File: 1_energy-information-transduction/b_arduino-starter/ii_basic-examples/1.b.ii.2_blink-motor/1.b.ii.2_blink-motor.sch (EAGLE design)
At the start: 2 parts, among them T1 2N706

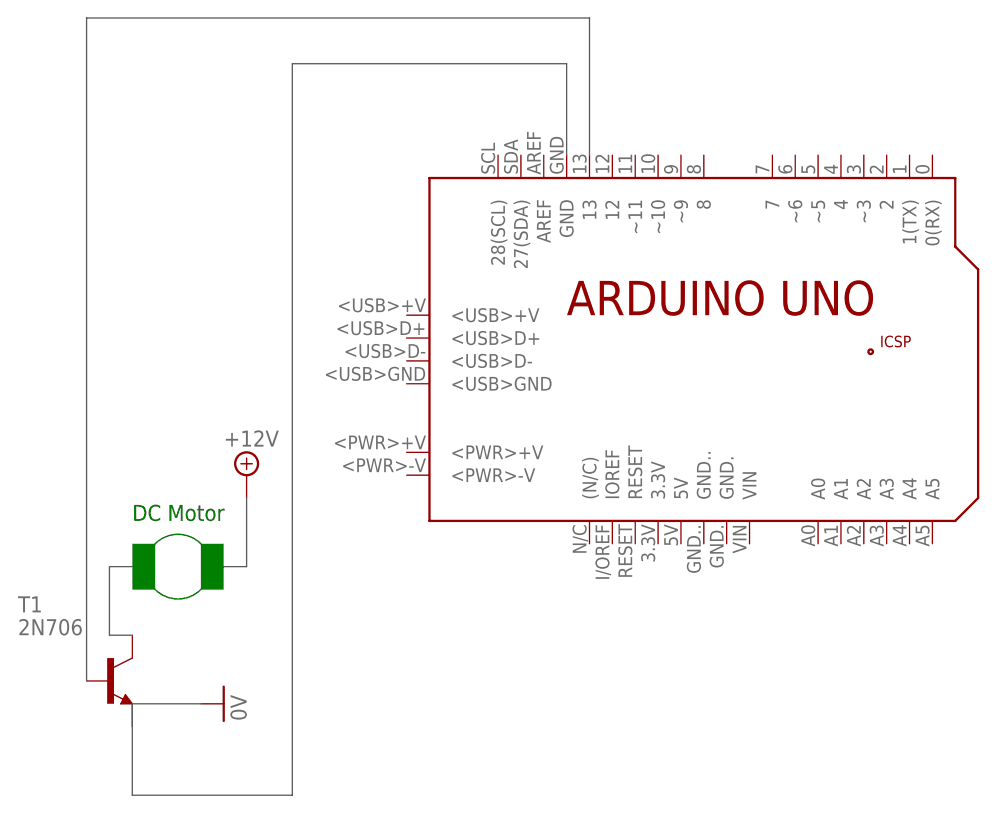
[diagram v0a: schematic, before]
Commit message: Bus to net.
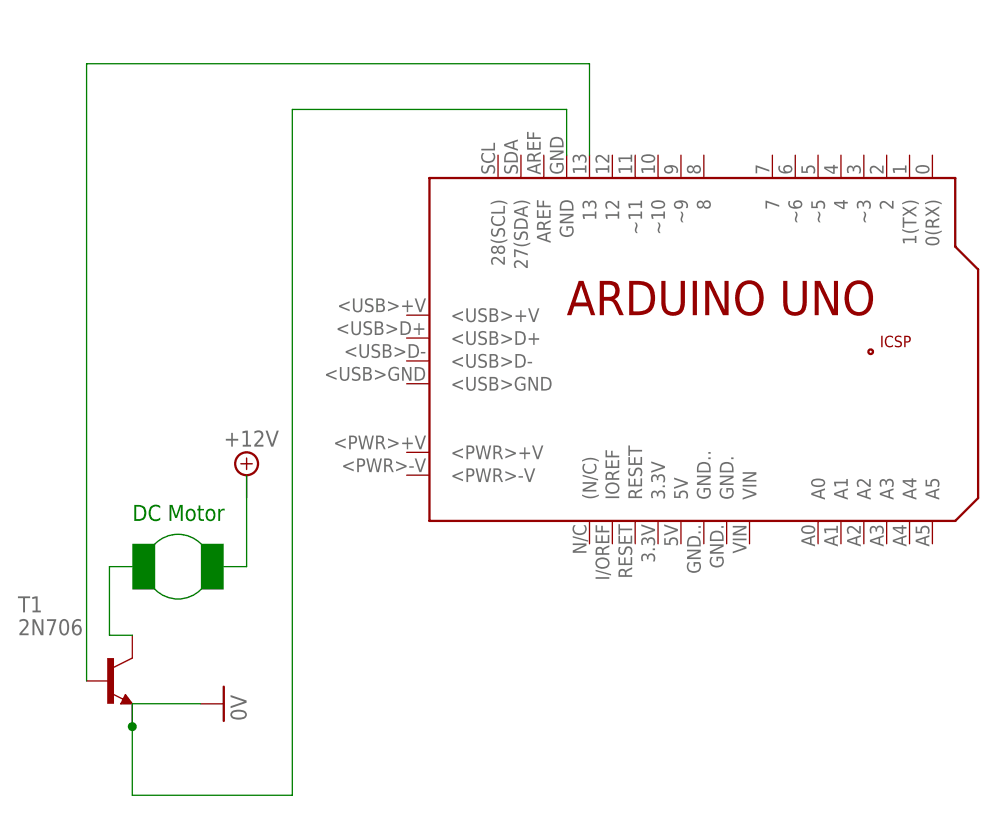
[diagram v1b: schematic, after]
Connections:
- new net 0V: PCB1.GND, T1.E
- new net N$2: T1.C
- new net N$3: PCB1.13, T1.B
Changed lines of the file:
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@@
 </instances>
 <busses>
-<bus name="B$2">
-<segment>
-<wire x1="93.98" y1="50.8" x2="93.98" y2="66.04" width="0.762" layer="92"/>
-<wire x1="93.98" y1="66.04" x2="38.1" y2="66.04" width="0.762" layer="92"/>
-<wire x1="38.1" y1="66.04" x2="38.1" y2="-7.62" width="0.762" layer="92"/>
-</segment>
-</bus>
-<bus name="B$3">
-<segment>
-<wire x1="91.44" y1="50.8" x2="91.44" y2="60.96" width="0.762" layer="92"/>
-<wire x1="91.44" y1="60.96" x2="60.96" y2="60.96" width="0.762" layer="92"/>
-<wire x1="60.96" y1="60.96" x2="60.96" y2="-20.32" width="0.762" layer="92"/>
-<wire x1="60.96" y1="-20.32" x2="43.18" y2="-20.32" width="0.762" layer="92"/>
-<wire x1="43.18" y1="-20.32" x2="43.18" y2="-10.16" width="0.762" layer="92"/>
-<wire x1="50.8" y1="-10.16" x2="43.18" y2="-10.16" width="0.762" layer="92"/>
-</segment>
-</bus>
-<bus name="B$4">
-<segment>
-<wire x1="43.18" y1="5.08" x2="40.64" y2="5.08" width="0.762" layer="92"/>
-<wire x1="40.64" y1="5.08" x2="40.64" y2="-2.54" width="0.762" layer="92"/>
-<wire x1="40.64" y1="-2.54" x2="43.18" y2="-2.54" width="0.762" layer="92"/>
-</segment>
-</bus>
-<bus name="B$5">
-<segment>
-<wire x1="55.88" y1="12.7" x2="55.88" y2="5.08" width="0.762" layer="92"/>
-<wire x1="55.88" y1="5.08" x2="53.34" y2="5.08" width="0.762" layer="92"/>
-</segment>
-</bus>
 </busses>
 <nets>
+<net name="N$1" class="0">
+<segment>
+<wire x1="53.34" y1="5.08" x2="55.88" y2="5.08" width="0.1524" layer="91"/>
+<wire x1="55.88" y1="5.08" x2="55.88" y2="15.24" width="0.1524" layer="91"/>
+</segment>
+</net>
+<net name="N$2" class="0">
+<segment>
+<wire x1="43.18" y1="5.08" x2="40.64" y2="5.08" width="0.1524" layer="91"/>
+<wire x1="40.64" y1="5.08" x2="40.64" y2="-2.54" width="0.1524" layer="91"/>
+<pinref part="T1" gate="G$1" pin="C"/>
+<wire x1="40.64" y1="-2.54" x2="43.18" y2="-2.54" width="0.1524" layer="91"/>
+</segment>
+</net>
+<net name="N$3" class="0">
+<segment>
+<pinref part="T1" gate="G$1" pin="B"/>
+<wire x1="38.1" y1="-7.62" x2="38.1" y2="60.96" width="0.1524" layer="91"/>
+<pinref part="PCB1" gate="G$1" pin="13"/>
+<wire x1="38.1" y1="60.96" x2="93.98" y2="60.96" width="0.1524" layer="91"/>
+<wire x1="93.98" y1="60.96" x2="93.98" y2="50.8" width="0.1524" layer="91"/>
+</segment>
+</net>
+<net name="0V" class="0">
+<segment>
+<pinref part="GND1" gate="1" pin="0V"/>
+<pinref part="T1" gate="G$1" pin="E"/>
+<wire x1="50.8" y1="-10.16" x2="43.18" y2="-10.16" width="0.1524" layer="91"/>
+<wire x1="43.18" y1="-10.16" x2="43.18" y2="-12.7" width="0.1524" layer="91"/>
+<wire x1="43.18" y1="-12.7" x2="43.18" y2="-20.32" width="0.1524" layer="91"/>
+<junction x="43.18" y="-12.7"/>
+<wire x1="43.18" y1="-20.32" x2="60.96" y2="-20.32" width="0.1524" layer="91"/>
+<wire x1="60.96" y1="-20.32" x2="60.96" y2="55.88" width="0.1524" layer="91"/>
+<pinref part="PCB1" gate="G$1" pin="GND"/>
+<wire x1="60.96" y1="55.88" x2="91.44" y2="55.88" width="0.1524" layer="91"/>
+<wire x1="91.44" y1="55.88" x2="91.44" y2="50.8" width="0.1524" layer="91"/>
+</segment>
+</net>
 </nets>
 </sheet>
